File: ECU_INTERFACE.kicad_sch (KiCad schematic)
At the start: 0 parts

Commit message: SCH Save
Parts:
- added J10: 5569-16A2, Connector_Molex:Molex_Mini-Fit_Jr_5569-16A2_2x08_P4.20mm_Horizontal, symbol Connector_Generic:Conn_02x08_Top_Bottom
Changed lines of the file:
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@@
 	(generator_version "10.0")
 	(paper "A4")
+	(symbol
+		(lib_id "Connector_Generic:Conn_02x08_Top_Bottom")
+		(at 74.93 59.69 0)
+		(mirror x)
+		(unit 1)
+		(body_style 1)
+		(exclude_from_sim no)
+		(in_bom yes)
+		(on_board yes)
+		(in_pos_files yes)
+		(dnp no)
+		(property "Reference" "J10"
+			(at 76.2 46.99 0)
+			(show_name no)
+			(do_not_autoplace no)
+			(effects
+				(font
+					(size 1.27 1.27)
+				)
+			)
+		)
+		(property "Value" "5569-16A2"
+			(at 76.2 69.85 0)
+			(show_name no)
+			(do_not_autoplace no)
+			(effects
+				(font
+					(size 1.27 1.27)
+				)
+			)
+		)
+		(property "Footprint" "Connector_Molex:Molex_Mini-Fit_Jr_5569-16A2_2x08_P4.20mm_Horizontal"
+			(at 74.93 59.69 0)
+			(hide yes)
+			(show_name no)
+			(do_not_autoplace no)
+			(effects
+				(font
+					(size 1.27 1.27)
+				)
+			)
+		)
+		(property "Datasheet" ""
+			(at 74.93 59.69 0)
+			(hide yes)
+			(show_name no)
+			(do_not_autoplace no)
+			(effects
+				(font
+					(size 1.27 1.27)
+				)
+			)
+		)
+		(property "Description" ""
+			(at 74.93 59.69 0)
+			(hide yes)
+			(show_name no)
+			(do_not_autoplace no)
+			(effects
+				(font
+					(size 1.27 1.27)
+				)
+			)
+		)
+		(property "LCSC" "C485577"
+			(at 74.93 59.69 0)
+			(hide yes)
+			(show_name no)
+			(do_not_autoplace no)
+			(effects
+				(font
+					(size 1.27 1.27)
+				)
+			)
+		)
+		(pin "1"
+		)
+		(pin "10"
+		)
+		(pin "11"
+		)
+		(pin "12"
+		)
+		(pin "13"
+		)
+		(pin "14"
+		)
+		(pin "15"
+		)
+		(pin "16"
+		)
+		(pin "2"
+		)
+		(pin "3"
+		)
+		(pin "4"
+		)
+		(pin "5"
+		)
+		(pin "6"
+		)
+		(pin "7"
+		)
+		(pin "8"
+		)
+		(pin "9"
+		)
+		(instances
+			(project "Hub-2.0"
+				(path "/af8ad92e-80c5-47c7-b528-865d82af0364/92353b5a-0bb5-4764-8ad6-9a983b2830ec"
+					(reference "J10")
+					(unit 1)
+				)
+			)
+		)
+	)
 )

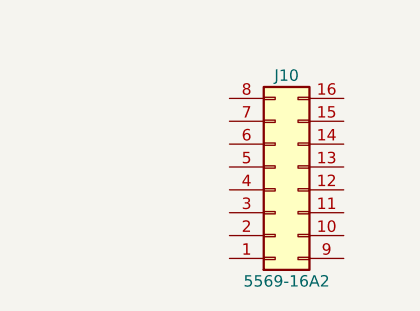
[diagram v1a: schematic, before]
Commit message: Autosave
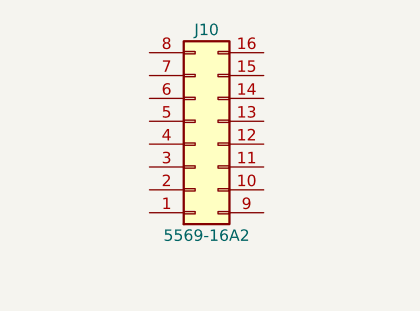
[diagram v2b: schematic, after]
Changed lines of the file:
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@@
 	(symbol
 		(lib_id "Connector_Generic:Conn_02x08_Top_Bottom")
-		(at 74.93 59.69 0)
+		(at 66.04 54.61 0)
 		(mirror x)
 		(unit 1)
@@
 		(dnp no)
 		(property "Reference" "J10"
-			(at 76.2 46.99 0)
+			(at 67.31 41.91 0)
 			(show_name no)
 			(do_not_autoplace no)
@@
 		)
 		(property "Value" "5569-16A2"
-			(at 76.2 69.85 0)
+			(at 67.31 64.77 0)
 			(show_name no)
 			(do_not_autoplace no)
@@
 		)
 		(property "Footprint" "Connector_Molex:Molex_Mini-Fit_Jr_5569-16A2_2x08_P4.20mm_Horizontal"
-			(at 74.93 59.69 0)
+			(at 66.04 54.61 0)
 			(hide yes)
 			(show_name no)
@@
 		)
 		(property "Datasheet" ""
-			(at 74.93 59.69 0)
+			(at 66.04 54.61 0)
 			(hide yes)
 			(show_name no)
@@
 		)
 		(property "Description" ""
-			(at 74.93 59.69 0)
+			(at 66.04 54.61 0)
 			(hide yes)
 			(show_name no)
@@
 		)
 		(property "LCSC" "C485577"
-			(at 74.93 59.69 0)
+			(at 66.04 54.61 0)
 			(hide yes)
 			(show_name no)

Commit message: Autosave
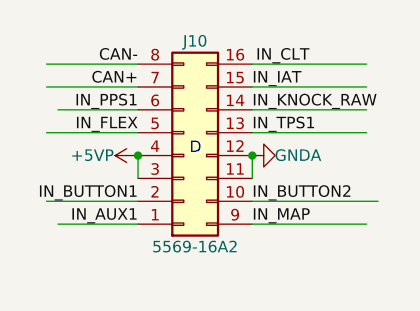
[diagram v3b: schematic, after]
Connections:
- net IN_AUX1: now reaches J10.1 (Pin_1)
- net IN_BUTTON2: now reaches J10.10 (Pin_10)
- net GNDA: now reaches J10.11 (Pin_11)
- net GNDA: now also J10.12 (Pin_12)
- net IN_TPS1: now reaches J10.13 (Pin_13)
- net IN_KNOCK_RAW: now reaches J10.14 (Pin_14)
- net IN_IAT: now reaches J10.15 (Pin_15)
- net IN_CLT: now reaches J10.16 (Pin_16)
- net IN_BUTTON1: now reaches J10.2 (Pin_2)
- net +5VP: now reaches J10.3 (Pin_3)
- net +5VP: now also J10.4 (Pin_4)
- net IN_FLEX: now reaches J10.5 (Pin_5)
- net IN_PPS1: now reaches J10.6 (Pin_6)
- net CAN+: now reaches J10.7 (Pin_7)
- net CAN-: now reaches J10.8 (Pin_8)
- net IN_MAP: now reaches J10.9 (Pin_9)
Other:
- note added: "D"
